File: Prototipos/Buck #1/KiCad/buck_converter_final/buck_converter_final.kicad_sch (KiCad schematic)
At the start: 24 parts, among them J3 Screw_Terminal_01x02, Q1 IRF9540NPBF, Q3 NPN

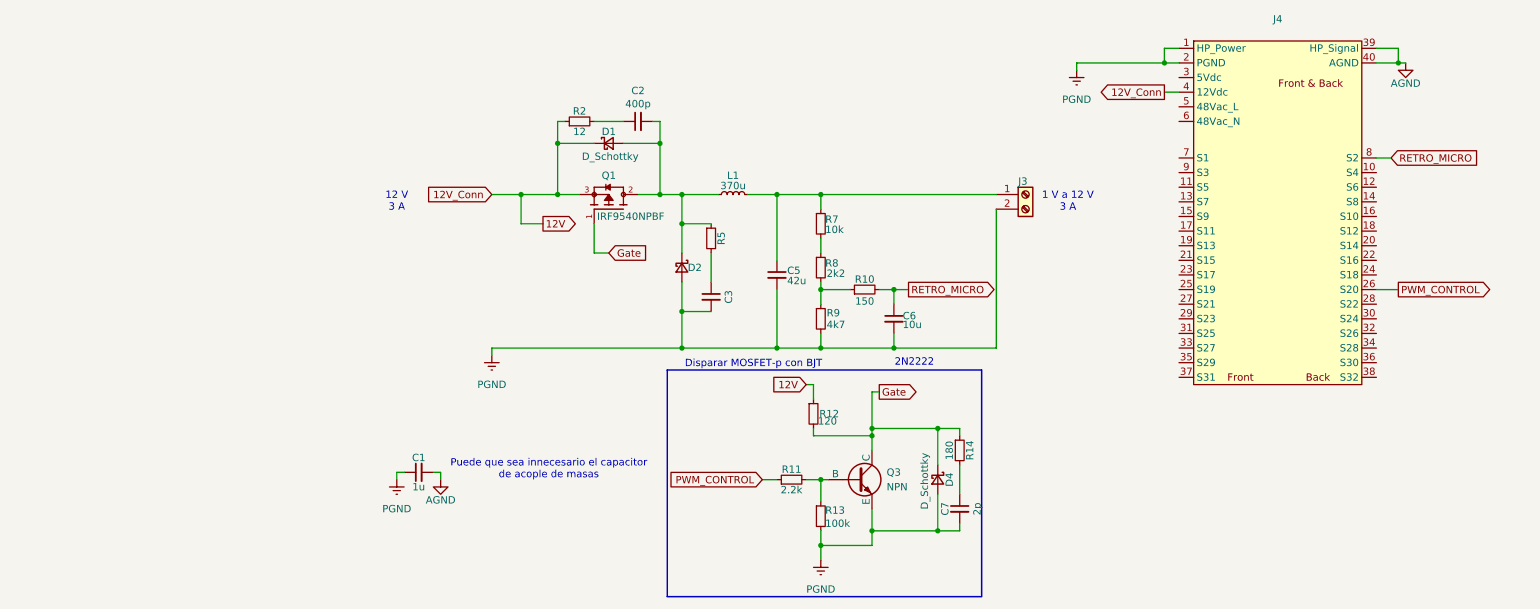
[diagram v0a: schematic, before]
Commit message: Reestructuración de esquemático y PCB
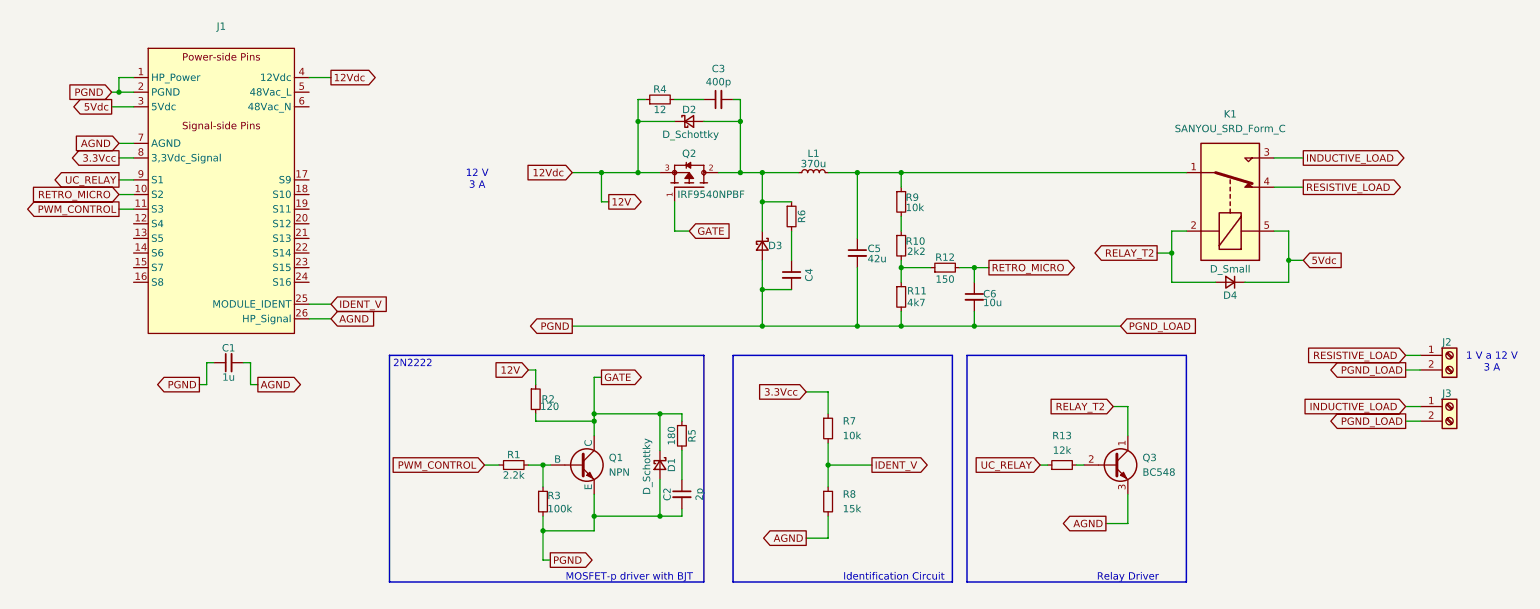
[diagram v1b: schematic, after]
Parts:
- removed J4: ~, Proyecto_Final:BUS_PCIE_x4_NSH, symbol Proyecto_Final:PCIE_x4_NSH
- added D4: D_Small, Diode_THT:D_DO-41_SOD81_P7.62mm_Horizontal, symbol Device:D_Small
- added J1: ~, Proyecto_final:BUS_PCIE_x4_NSH, symbol Proyecto_Final:PCIE_x4_NSH
- added J3: Screw_Terminal_01x02, TerminalBlock_Phoenix:TerminalBlock_Phoenix_MKDS-1,5-2-5.08_1x02_P5.08mm_Horizontal, symbol Connector:Screw_Terminal_01x02
- added K1: SANYOU_SRD_Form_C, Relay_THT:Relay_SPDT_SANYOU_SRD_Series_Form_C, symbol Relay:SANYOU_SRD_Form_C
- added Q3: BC548, Package_TO_SOT_THT:TO-92_Inline_Wide, symbol Transistor_BJT:BC548
- added R13: 12k, Resistor_THT:R_Axial_DIN0207_L6.3mm_D2.5mm_P7.62mm_Horizontal, symbol Device:R_Small
- added R7: 10k, Resistor_THT:R_Axial_DIN0207_L6.3mm_D2.5mm_P7.62mm_Horizontal, symbol Device:R_Small
- added R8: 15k, Resistor_THT:R_Axial_DIN0207_L6.3mm_D2.5mm_P7.62mm_Horizontal, symbol Device:R_Small
- renumbered C7 to C2, C2 to C3, C3 to C4, D4 to D1, D1 to D2, D2 to D3, J3 to J2, Q3 to Q1, Q1 to Q2, R11 to R1, R8 to R10, R9 to R11, R10 to R12, R12 to R2, R13 to R3, R2 to R4, R14 to R5, R5 to R6, R7 to R9
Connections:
- net 12V: now also J1.4 (12Vdc)
- net AGND: now also J1.26 (HP_Signal), J1.7 (AGND), Q3.3 (E), R8.2
- net PGND: now also J1.1 (HP_Power), J1.2 (PGND), J3.2 (Pin_2)
- net PWM_CONTROL: now also J1.11 (S3)
- net RETRO_MICRO: now also J1.10 (S2)
- net at C5.1, L1.2, R9.1: now also K1.1; no longer J2.1 (Pin_1)
- net Gate renamed GATE
- new net: Q3.2 (B), R13.2
- new net 3.3Vcc: J1.8 (3,3Vdc_Signal), R7.1
- new net 5Vdc: D4.1 (K), J1.3 (5Vdc), K1.5
- new net IDENT_V: J1.25 (MODULE_IDENT), R7.2, R8.1
- new net INDUCTIVE_LOAD: J3.1 (Pin_1), K1.3
- new net RELAY_T2: D4.2 (A), K1.2, Q3.1 (C)
- new net RESISTIVE_LOAD: J2.1 (Pin_1), K1.4
- new net UC_RELAY: J1.9 (S1), R13.1
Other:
- note added: "Identification Circuit"
- note added: "MOSFET-p driver with BJT"
- note added: "Relay Driver"
- note removed: "Disparar MOSFET-p con BJT"
- note removed: "Puede que sea innecesario el capacitor de acople de masas"
- moved on the sheet: C1, C2, C3, C4, C5, C6, D1, D2, D3, J2, L1, Q1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

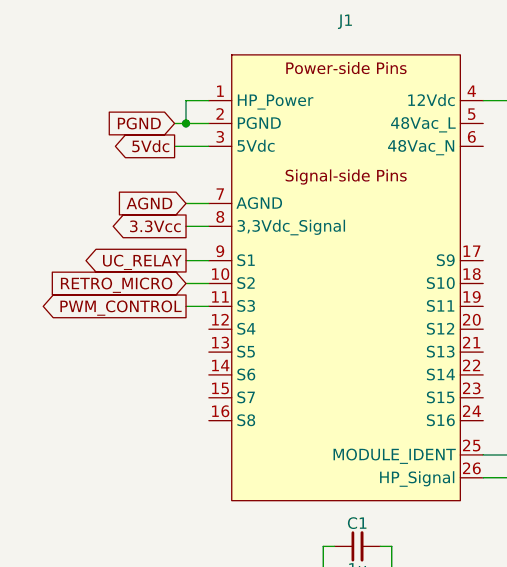
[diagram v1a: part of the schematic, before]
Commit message: Avances en PCB buck
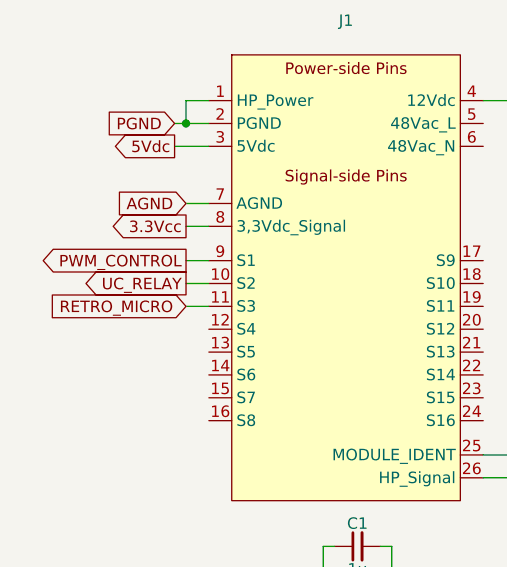
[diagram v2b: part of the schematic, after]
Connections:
- net PWM_CONTROL: now also J1.9 (S1); no longer J1.11 (S3)
- net RETRO_MICRO: now also J1.11 (S3); no longer J1.10 (S2)
- net UC_RELAY: now also J1.10 (S2); no longer J1.9 (S1)
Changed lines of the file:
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@@
+	(wire
+		(pts
+			(xy 35.56 54.61) (xy 38.1 54.61)
+		)
+		(stroke
+			(width 0)
+			(type default)
+		)
+	)
 	(wire
 		(pts
@@
 	(wire
 		(pts
+			(xy 35.56 52.07) (xy 38.1 52.07)
+		)
+		(stroke
+			(width 0)
+			(type default)
+		)
+	)
+	(wire
+		(pts
 			(xy 158.75 97.79) (xy 158.75 101.6)
 		)
@@
 	(wire
 		(pts
-			(xy 35.56 52.07) (xy 38.1 52.07)
-		)
-		(stroke
-			(width 0)
-			(type default)
-		)
-	)
-	(wire
-		(pts
 			(xy 186.69 67.31) (xy 184.15 67.31)
 		)
@@
 		(pts
 			(xy 49.53 87.63) (xy 50.8 87.63)
-		)
-		(stroke
-			(width 0)
-			(type default)
-		)
-	)
-	(wire
-		(pts
-			(xy 35.56 54.61) (xy 38.1 54.61)
 		)
 		(stroke
@@
 	(global_label "RETRO_MICRO"
 		(shape input)
-		(at 35.56 54.61 180)
-		(fields_autoplaced yes)
-		(effects
-			(font
-				(size 1.27 1.27)
-			)
-			(justify right)
-		)
-		(property "Intersheetrefs" "${INTERSHEET_REFS}"
-			(at 19.6934 54.61 0)
+		(at 35.56 57.15 180)
+		(fields_autoplaced yes)
+		(effects
+			(font
+				(size 1.27 1.27)
+			)
+			(justify right)
+		)
+		(property "Intersheetrefs" "${INTERSHEET_REFS}"
+			(at 19.6934 57.15 0)
 			(effects
 				(font
@@
 	(global_label "PWM_CONTROL"
 		(shape output)
-		(at 35.56 57.15 180)
-		(fields_autoplaced yes)
-		(effects
-			(font
-				(size 1.27 1.27)
-			)
-			(justify right)
-		)
-		(property "Intersheetrefs" "${INTERSHEET_REFS}"
-			(at 18.9072 57.15 0)
+		(at 35.56 52.07 180)
+		(fields_autoplaced yes)
+		(effects
+			(font
+				(size 1.27 1.27)
+			)
+			(justify right)
+		)
+		(property "Intersheetrefs" "${INTERSHEET_REFS}"
+			(at 18.9072 52.07 0)
 			(effects
 				(font
@@
 	(global_label "UC_RELAY"
 		(shape output)
-		(at 35.56 52.07 180)
-		(fields_autoplaced yes)
-		(effects
-			(font
-				(size 1.27 1.27)
-			)
-			(justify right)
-		)
-		(property "Intersheetrefs" "${INTERSHEET_REFS}"
-			(at 23.3824 52.07 0)
-			(effects
-				(font
+		(at 35.56 54.61 180)
+		(fields_autoplaced yes)
+		(effects
+			(font
+				(size 1.27 1.27)
+			)
+			(justify right)
+		)
+		(property "Intersheetrefs" "${INTERSHEET_REFS}"
+			(at 23.3824 54.61 0)
+			(effects
+				(font
